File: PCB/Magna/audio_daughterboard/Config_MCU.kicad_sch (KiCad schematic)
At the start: 1 part, among them U1401 STM32F030C8Tx

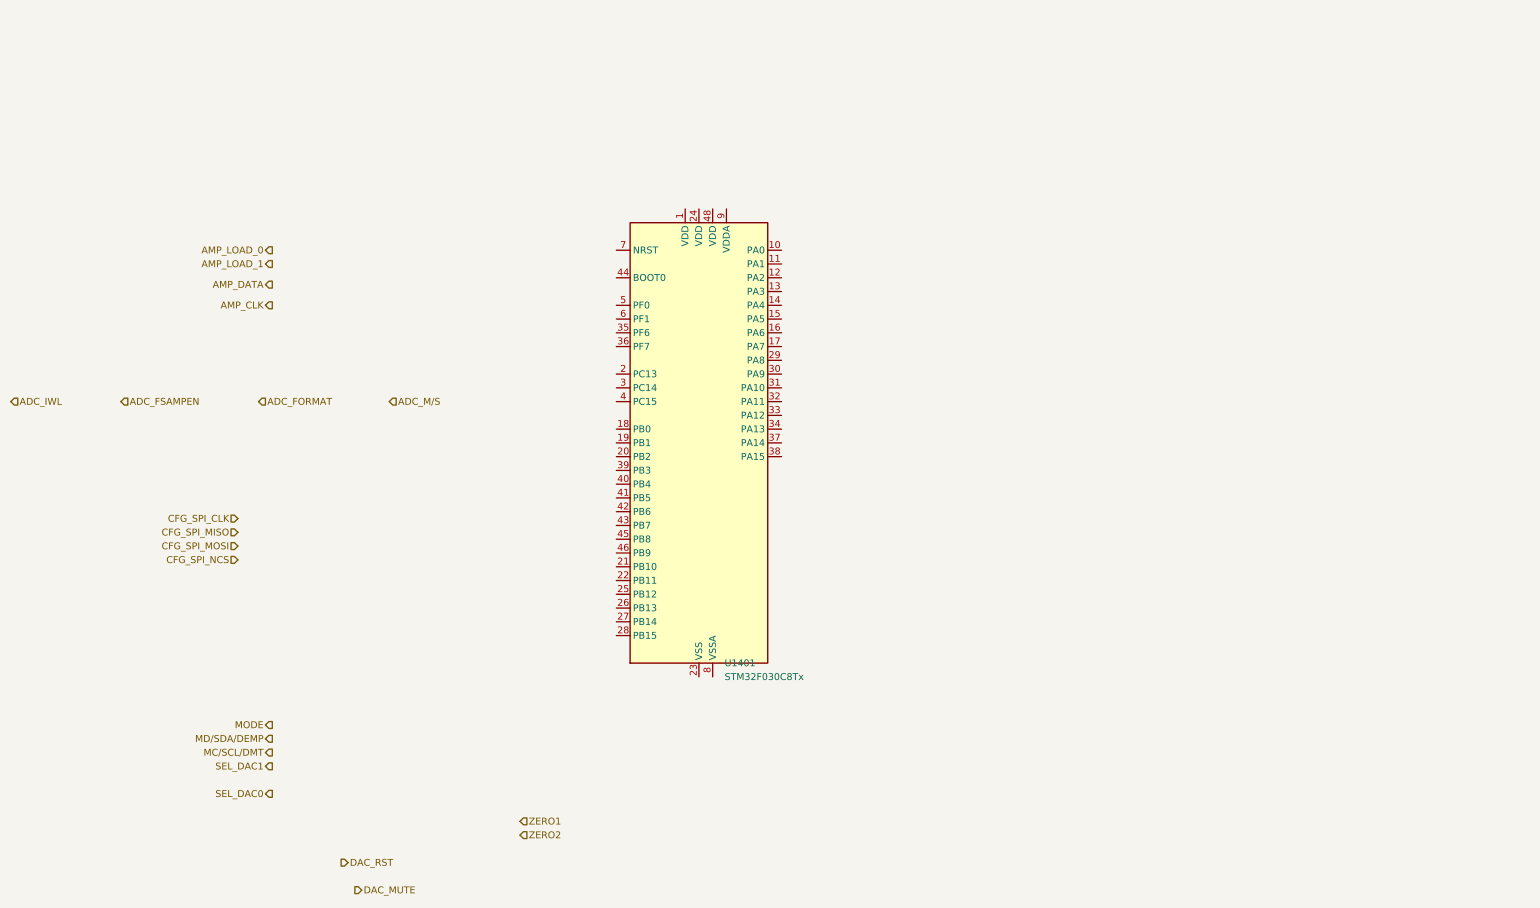
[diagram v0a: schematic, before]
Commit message: "Finalize" Audio daugherboard
Finished DAC output filter
Fixed the whole damn MCU subschematic
Fixed Linedriver schematic
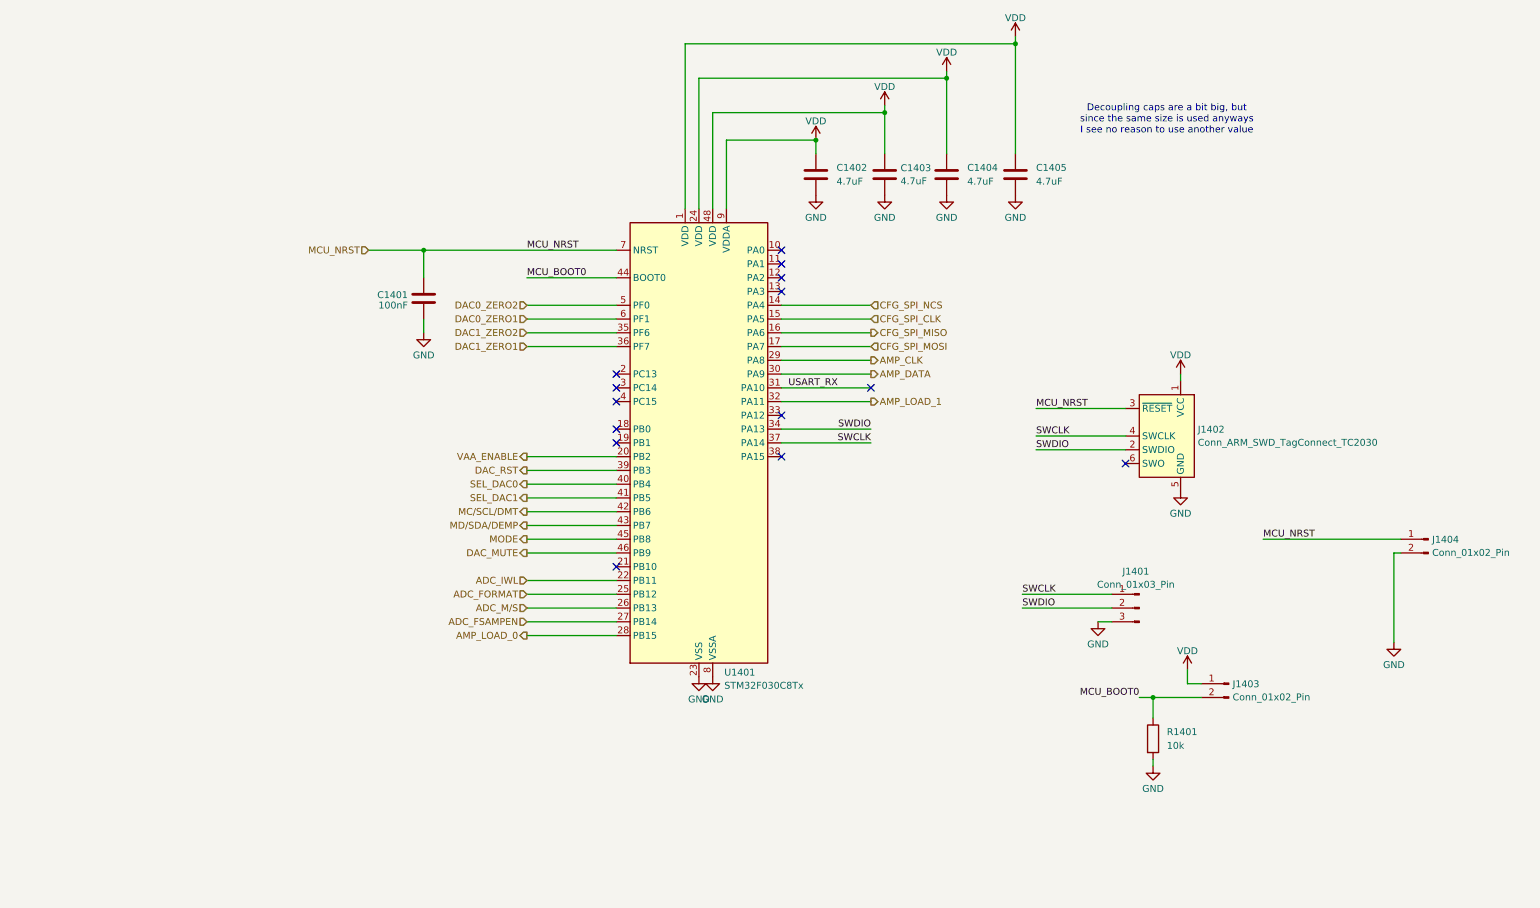
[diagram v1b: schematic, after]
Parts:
- added C1401: 100nF, Capacitor_SMD:C_0805_2012Metric_Pad1.18x1.45mm_HandSolder, symbol Device:C
- added C1402, C1403, C1404, C1405: 4.7uF, Capacitor_SMD:C_0805_2012Metric_Pad1.18x1.45mm_HandSolder, symbol Device:C
- added J1401: Conn_01x03_Pin, symbol Connector:Conn_01x03_Pin
- added J1402: Conn_ARM_SWD_TagConnect_TC2030, Connector:Tag-Connect_TC2030-IDC-FP_2x03_P1.27mm_Vertical, symbol Connector:Conn_ARM_SWD_TagConnect_TC2030
- added J1403, J1404: Conn_01x02_Pin, symbol Connector:Conn_01x02_Pin
- added R1401: 10k, Resistor_SMD:R_0805_2012Metric_Pad1.20x1.40mm_HandSolder, symbol Device:R
- U1401: symbol MCU_ST_STM32F0:STM32F030C8Tx -> MCU_ST_STM32F0:STM32F030C6Tx
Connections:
- net ADC_FORMAT: now also U1401.25 (PB12)
- net ADC_FSAMPEN: now also U1401.27 (PB14)
- net ADC_IWL: now also U1401.22 (PB11)
- net ADC_M/S: now also U1401.26 (PB13)
- net AMP_CLK: now also U1401.29 (PA8)
- net AMP_DATA: now also U1401.30 (PA9)
- net AMP_LOAD_0: now also U1401.28 (PB15)
- net AMP_LOAD_1: now also U1401.32 (PA11)
- net CFG_SPI_CLK: now also U1401.15 (PA5)
- net CFG_SPI_MISO: now also U1401.16 (PA6)
- net CFG_SPI_MOSI: now also U1401.17 (PA7)
- net CFG_SPI_NCS: now also U1401.14 (PA4)
- net DAC_MUTE: now also U1401.46 (PB9)
- net DAC_RST: now also U1401.39 (PB3)
- net MC/SCL/DMT: now also U1401.42 (PB6)
- net MD/SDA/DEMP: now also U1401.43 (PB7)
- net MODE: now also U1401.45 (PB8)
- net SEL_DAC0: now also U1401.40 (PB4)
- net SEL_DAC1: now also U1401.41 (PB5)
- net VDD: now reaches U1401.1 (VDD)
- net VDD: now also U1401.24 (VDD), U1401.48 (VDD), U1401.9 (VDDA), C1402.1, C1403.1, C1404.1, C1405.1, J1402.1 (VCC), J1403.1 (Pin_1)
- net VAA_ENABLE: now reaches U1401.20 (PB2)
- net GND: now reaches U1401.23 (VSS), U1401.47 (VSS)
- net GND: now also U1401.8 (VSSA), C1401.2, C1402.2, C1403.2, C1404.2, C1405.2, J1401.3 (Pin_3), J1402.5 (GND), J1404.2 (Pin_2), R1401.2
- net USART_RX: now reaches U1401.31 (PA10)
- net SWDIO: now reaches U1401.34 (PA13)
- net SWDIO: now also J1401.2 (Pin_2), J1402.2 (SWDIO)
- net DAC1_ZERO2: now reaches U1401.35 (PF6)
- net DAC1_ZERO1: now reaches U1401.36 (PF7)
- net SWCLK: now reaches U1401.37 (PA14)
- net SWCLK: now also J1401.1 (Pin_1), J1402.4 (SWCLK)
- net MCU_BOOT0: now reaches U1401.44 (BOOT0)
- net MCU_BOOT0: now also J1403.2 (Pin_2), R1401.1
- net DAC0_ZERO2: now reaches U1401.5 (PF0)
- net DAC0_ZERO1: now reaches U1401.6 (PF1)
- net MCU_NRST: now reaches U1401.7 (NRST)
- net MCU_NRST: now also C1401.1, J1402.3 (~{RESET}), J1404.1 (Pin_1)
- no-connect marks 0 -> 14
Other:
- note added: "Decoupling caps are a bit big, but since the same size is used anyways I see no reason to use another value"
